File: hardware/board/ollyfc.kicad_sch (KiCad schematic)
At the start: 63 parts, among them CN1 20021521-00010T1LF, J1 Conn_01x06, J12 Conn_01x08, J13 Conn_01x04, J4 Conn_01x06, Q2 MMBT3904, Q3 MMBT3904, SW2 SW_Push, SW3 SW_Push, SW5 MODE1, U3 STM32F411RETx, U6 W25Q128JVS, X1 X322516MLB4SI

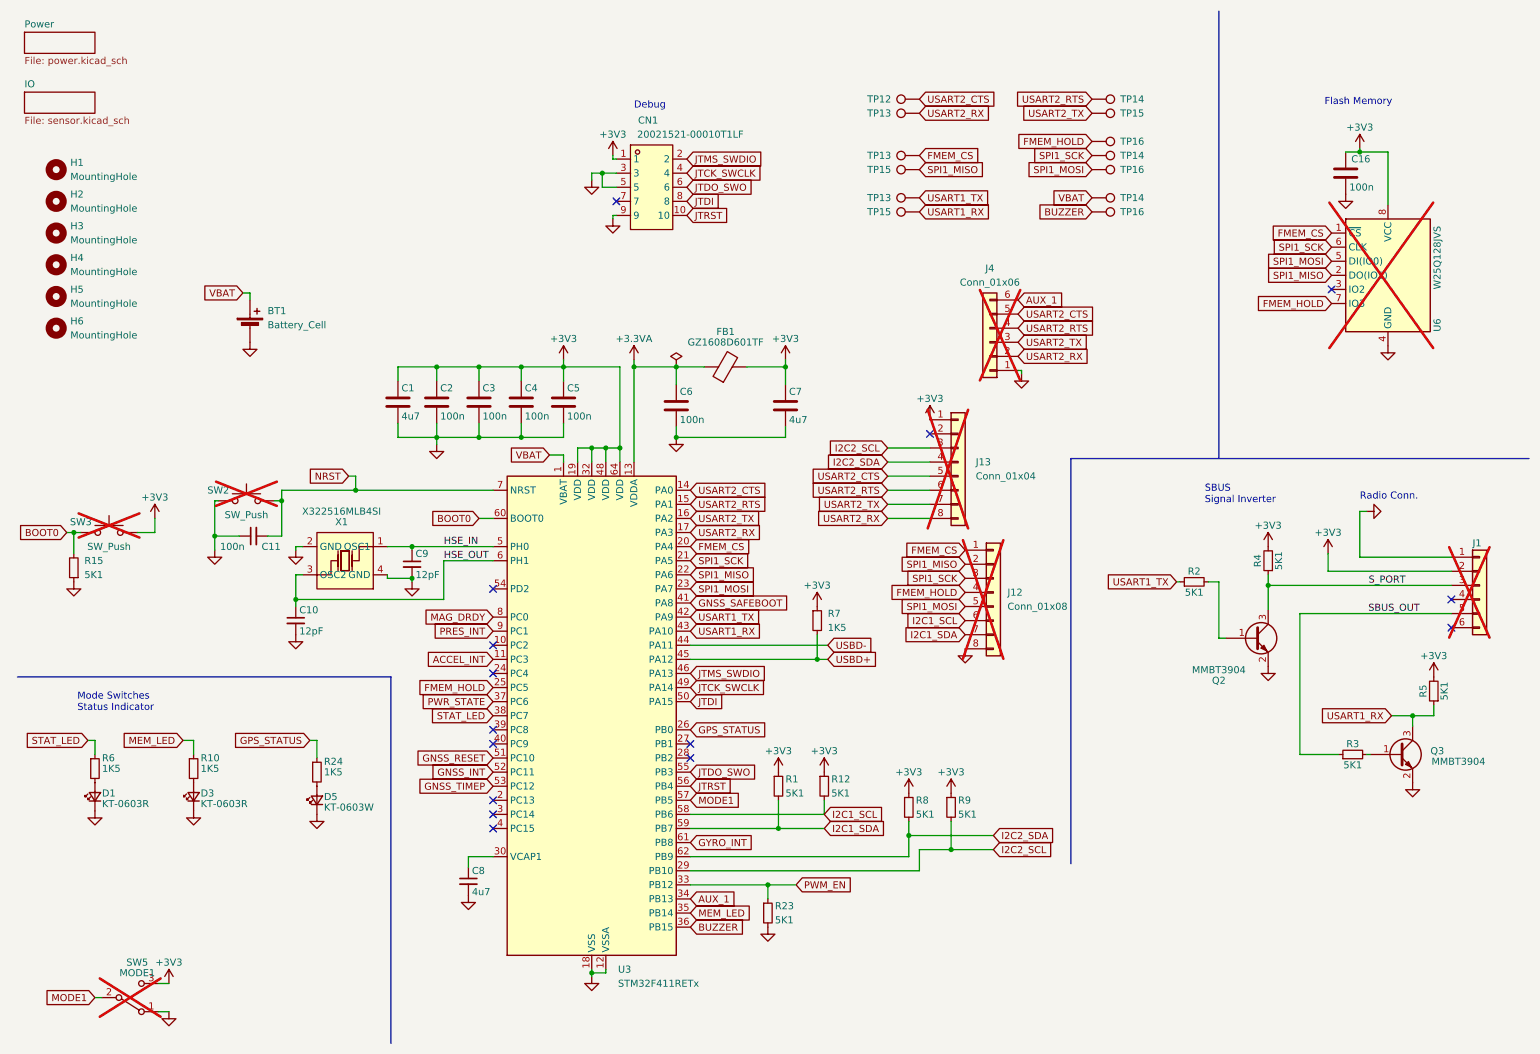
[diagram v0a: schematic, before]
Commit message: v3 schematic + layout
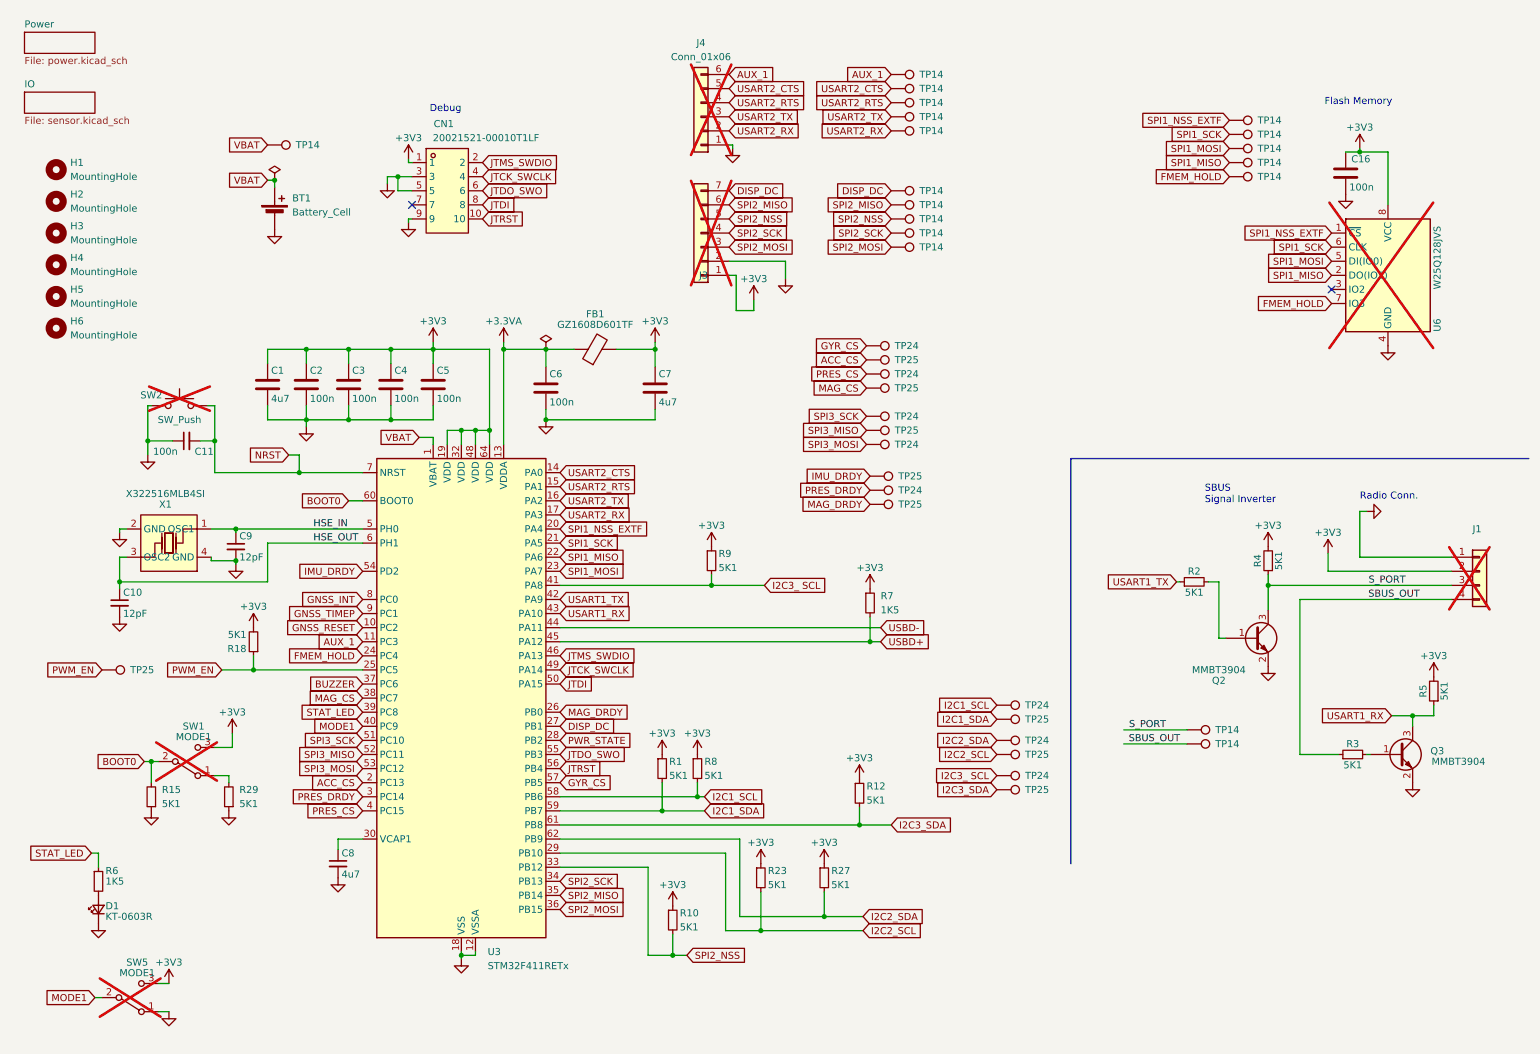
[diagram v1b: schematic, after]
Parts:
- removed D3: KT-0603R, LED_SMD:LED_0603_1608Metric, symbol Device:LED_Small
- removed D5: KT-0603W, LED_SMD:LED_0603_1608Metric, symbol Device:LED_Small
- removed J1: Conn_01x06, Connector_JST:JST_PH_B6B-PH-K_1x06_P2.00mm_Vertical, symbol Connector_Generic:Conn_01x06
- removed J12: Conn_01x08, Connector_PinHeader_2.54mm:PinHeader_1x08_P2.54mm_Vertical, symbol Connector_Generic:Conn_01x08
- removed J13: Conn_01x04, Connector_PinHeader_2.54mm:PinHeader_1x08_P2.54mm_Vertical, symbol Connector_Generic:Conn_01x08
- removed R24: 1K5, Resistor_SMD:R_0402_1005Metric, symbol Device:R_Small
- removed SW3: SW_Push, Button_Switch_THT:SW_PUSH_6mm, symbol Switch:SW_Push
- removed TP12, TP13 (x3), TP14 (x2), TP15 (x3), TP16 (x3): TestPoint, TestPoint:TestPoint_Pad_D1.5mm, symbol Connector:TestPoint
- added J1: Conn_01x04, Connector_JST:JST_PH_B4B-PH-K_1x04_P2.00mm_Vertical, symbol Connector_Generic:Conn_01x04
- added J3: Conn_01x07, Connector_JST:JST_PH_B7B-PH-K_1x07_P2.00mm_Vertical, symbol Connector_Generic:Conn_01x07
- added R18, R27, R29: 5K1, Resistor_SMD:R_0402_1005Metric, symbol Device:R_Small
- added SW1: MODE1, Button_Switch_SMD:SW_SPDT_PCM12, symbol Switch:SW_SPDT
- added TP14 (x17), TP24 (x8), TP25 (x9): TestPoint, TestPoint:TestPoint_Pad_D1.0mm, symbol Connector:TestPoint
- R10: value 1K5 -> 5K1
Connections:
- net ACCEL_INT is gone; now on net AUX_1: U3.11 (PC3)
- net GPS_STATUS is gone; now on net MAG_DRDY: U3.26 (PB0)
- net PRES_INT is gone; now on net GNSS_TIMEP: U3.9 (PC1)
- net +3V3: now also R10.1, R23.1, J1.2 (Pin_2), J3.1 (Pin_1), R18.2, R27.1, SW1.3 (C)
- net AUX_1: now also TP14.1; no longer U3.34 (PB13)
- net BOOT0: now also SW1.2 (B)
- net BUZZER: now also U3.37 (PC6); no longer U3.36 (PB15)
- net FMEM_HOLD: now also U3.24 (PC4), TP14.1; no longer U3.25 (PC5)
- net GND: now also J1.1 (Pin_1), J3.2 (Pin_2), R29.1; no longer R23.2
- net GNSS_INT: now also U3.8 (PC0); no longer U3.52 (PC11)
- net GNSS_RESET: now also U3.10 (PC2); no longer U3.51 (PC10)
- net GNSS_TIMEP: no longer U3.53 (PC12)
- net I2C1_SCL: now also R8.2, TP24.1; no longer R12.2
- net I2C1_SDA: now also TP25.1
- net I2C2_SCL: now also R23.2, TP25.1; no longer R9.2
- net I2C2_SDA: now also R27.2, TP24.1; no longer R8.2
- net MAG_DRDY: now also TP25.1; no longer U3.8 (PC0)
- net MODE1: now also U3.40 (PC9); no longer U3.57 (PB5)
- net PWM_EN: now also U3.25 (PC5), R18.1, TP25.1; no longer R23.1, U3.33 (PB12)
- net PWR_STATE: now also U3.28 (PB2); no longer U3.37 (PC6)
- net SBUS_OUT: now also J1.4 (Pin_4), TP14.1
- net SPI1_MISO: now also TP14.1
- net SPI1_MOSI: now also TP14.1
- net SPI1_SCK: now also TP14.1
- net STAT_LED: now also U3.39 (PC8); no longer U3.38 (PC7)
- net S_PORT: now also J1.3 (Pin_3), TP14.1
- net USART2_CTS: now also TP14.1
- net USART2_RTS: now also TP14.1
- net USART2_RX: now also TP14.1
- net USART2_TX: now also TP14.1
- net ACC_CS: now reaches U3.2 (PC13)
- net ACC_CS: now also TP25.1
- net DISP_DC: now reaches U3.27 (PB1)
- net DISP_DC: now also J3.7 (Pin_7), TP14.1
- net PRES_DRDY: now reaches U3.3 (PC14)
- net PRES_DRDY: now also TP24.1
- net PRES_CS: now reaches U3.4 (PC15)
- net PRES_CS: now also TP24.1
- net IMU_DRDY: now reaches U3.54 (PD2)
- net IMU_DRDY: now also TP25.1
- net SPI2_NSS: now reaches R10.2
- net SPI2_NSS: now also U3.33 (PB12), J3.5 (Pin_5), TP14.1
- net FMEM_CS renamed SPI1_NSS_EXTF
- net SPI1_NSS_EXTF: now also TP14.1
- net GNSS_SAFEBOOT renamed I2C3_ SCL
- net I2C3_ SCL: now also R9.2, TP24.1
- net GYRO_INT renamed I2C3_SDA
- net I2C3_SDA: now also R12.2, TP25.1
- net MEM_LED renamed SPI2_MISO
- net SPI2_MISO: now also J3.6 (Pin_6), TP14.1; no longer R10.1
- new net: R29.2, SW1.1 (A)
- new net GYR_CS: TP24.1, U3.57 (PB5)
- new net MAG_CS: TP25.1, U3.38 (PC7)
- new net SPI2_MOSI: J3.3 (Pin_3), TP14.1, U3.36 (PB15)
- new net SPI2_SCK: J3.4 (Pin_4), TP14.1, U3.34 (PB13)
- new net SPI3_MISO: TP25.1, U3.52 (PC11)
- new net SPI3_MOSI: TP24.1, U3.53 (PC12)
- new net SPI3_SCK: TP24.1, U3.51 (PC10)
- no-connect marks 15 -> 2
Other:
- note removed: "Mode Switches Status Indicator"
- moved on the sheet: BT1, C1, C10, C11, C2, C3, C4, C5, C6, C7, C8, C9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
